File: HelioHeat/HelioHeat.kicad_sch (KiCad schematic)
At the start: 9 parts, among them U1 ATtiny85-20P, U2 CD4511BE, U3 CD4511BE, U4 CD4511BE, U5 74HC595, U6 74HC595

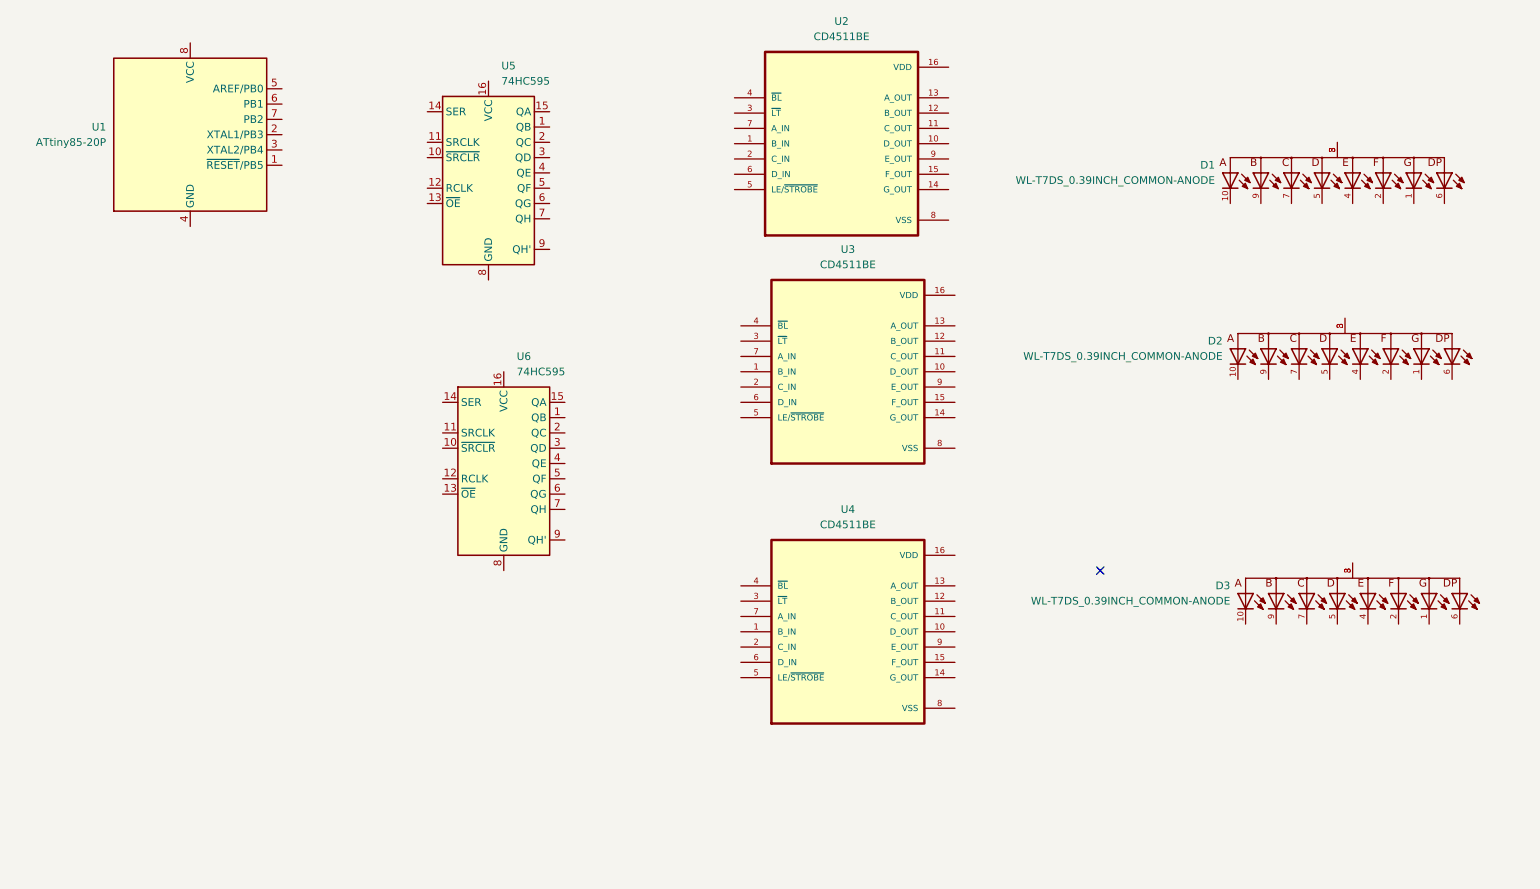
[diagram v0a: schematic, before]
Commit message: cables
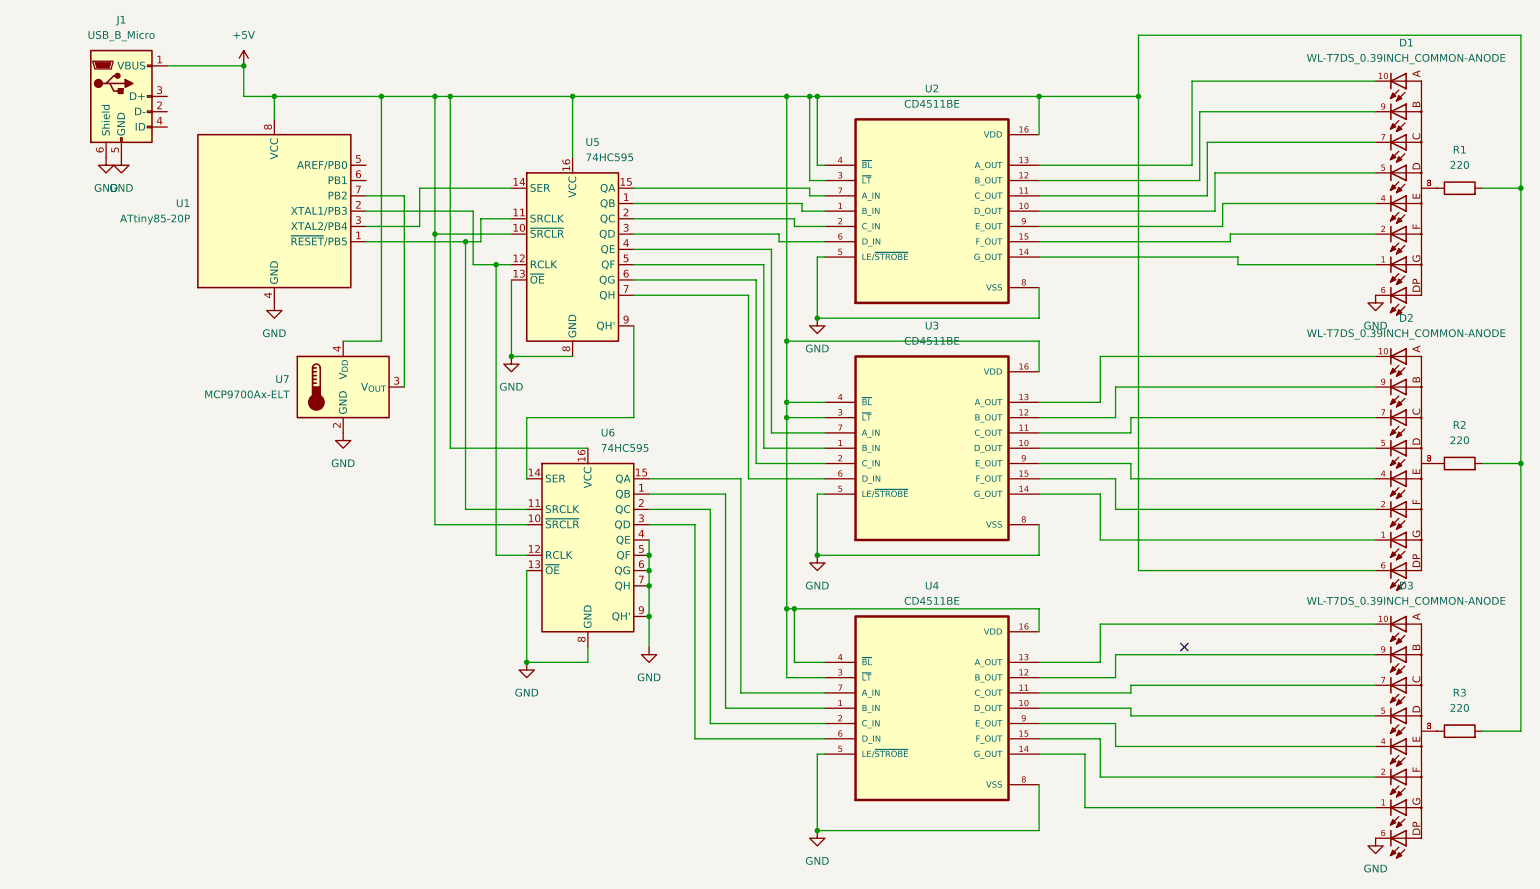
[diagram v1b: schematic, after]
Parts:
- added J1: USB_B_Micro, Connector_USB:USB_Micro-B_Amphenol_10103594-0001LF_Horizontal, symbol Connector:USB_B_Micro
- added R1, R2, R3: 220, Resistor_SMD:R_0201_0603Metric, symbol Device:R
- added U7: MCP9700Ax-ELT, Package_TO_SOT_SMD:SOT-353_SC-70-5, symbol Sensor_Temperature:MCP9700Ax-ELT
- U5, U6: footprint (none) -> 74HC595:SO16
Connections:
- net at U2.1 (B_IN): now also U5.1 (QB)
- net at U2.10 (D_OUT): now also D1.5
- net at U2.11 (C_OUT): now also D1.7
- net at U2.12 (B_OUT): now also D1.9
- net at U2.13 (A_OUT): now also D1.10
- net at U2.14 (G_OUT): now also D1.1
- net at U2.15 (F_OUT): now also D1.2
- net +5V: now reaches U2.16 (VDD)
- net +5V: now also D2.6, U1.8 (VCC), U2.3 (~{LT}), U2.4 (~{BL}), U3.16 (VDD), U3.3 (~{LT}), U3.4 (~{BL}), U4.16 (VDD), U4.3 (~{LT}), U4.4 (~{BL}), U5.10 (~{SRCLR}), U5.16 (VCC), U6.10 (~{SRCLR}), U6.16 (VCC), J1.1 (VBUS), R1.2, R2.2, R3.2, U7.4 (V_{DD})
- net at U2.2 (C_IN): now also U5.2 (QC)
- net GND: now reaches U2.5 (LE/~{STROBE})
- net GND: now also D1.6, D3.6, U1.4 (GND), U2.8 (VSS), U3.5 (LE/~{STROBE}), U3.8 (VSS), U4.5 (LE/~{STROBE}), U4.8 (VSS), U5.13 (~{OE}), U5.8 (GND), U6.13 (~{OE}), U6.4 (QE), U6.5 (QF), U6.6 (QG), U6.7 (QH), U6.8 (GND), U6.9 (QH'), J1.5 (GND), J1.6 (Shield), U7.2 (GND)
- net at U2.6 (D_IN): now also U5.3 (QD)
- net at U2.7 (A_IN): now also U5.15 (QA)
- net at U2.9 (E_OUT): now also D1.4
- net at U3.1 (B_IN): now also U5.5 (QF)
- net at U3.10 (D_OUT): now also D2.5
- net at U3.11 (C_OUT): now also D2.7
- net at U3.12 (B_OUT): now also D2.9
- net at U3.13 (A_OUT): now also D2.10
- net at U3.14 (G_OUT): now also D2.1
- net at U3.15 (F_OUT): now also D2.2
- net at U3.2 (C_IN): now also U5.6 (QG)
- net at U3.6 (D_IN): now also U5.7 (QH)
- net at U3.7 (A_IN): now also U5.4 (QE)
- net at U3.9 (E_OUT): now also D2.4
- net at U6.1 (QB): now also U4.1 (B_IN)
- net at U6.11 (SRCLK): now also U1.1 (~{RESET}/PB5), U5.11 (SRCLK)
- net at U6.12 (RCLK): now also U1.2 (XTAL1/PB3), U5.12 (RCLK)
- net at U6.14 (SER): now also U5.9 (QH')
- net at U6.15 (QA): now also U4.7 (A_IN)
- net at U6.2 (QC): now also U4.2 (C_IN)
- net at U6.3 (QD): now also U4.6 (D_IN)
- net at U5.14 (SER): now also U1.3 (XTAL2/PB4)
- net at D2.3, D2.8: now also R2.1
- net at D1.3, D1.8: now also R1.1
- net at D3.1: now also U4.14 (G_OUT)
- net at D3.10: now also U4.13 (A_OUT)
- net at D3.2: now also U4.15 (F_OUT)
- net at D3.3, D3.8: now also R3.1
- net at D3.4: now also U4.9 (E_OUT)
- net at D3.5: now also U4.10 (D_OUT)
- net at D3.7: now also U4.11 (C_OUT)
- net at D3.9: now also U4.12 (B_OUT)
- net at U1.7 (PB2): now also U7.3 (V_{OUT})
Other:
- moved on the sheet: D1, D2, D3, U1, U2, U3, U4, U5, U6
